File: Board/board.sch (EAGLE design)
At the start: 58 parts, among them IC1 L297, IC2 MEGA32-P, J1 +12V, Q1 BC639, Q2 BC639, Q3 BS170, Q4 BS170, Q5 BS170, Q6 BS170, X1 WATER_PUMP, X2 FAN, X3 STEP_MOT_CD, X4 STEP_MOT_AB

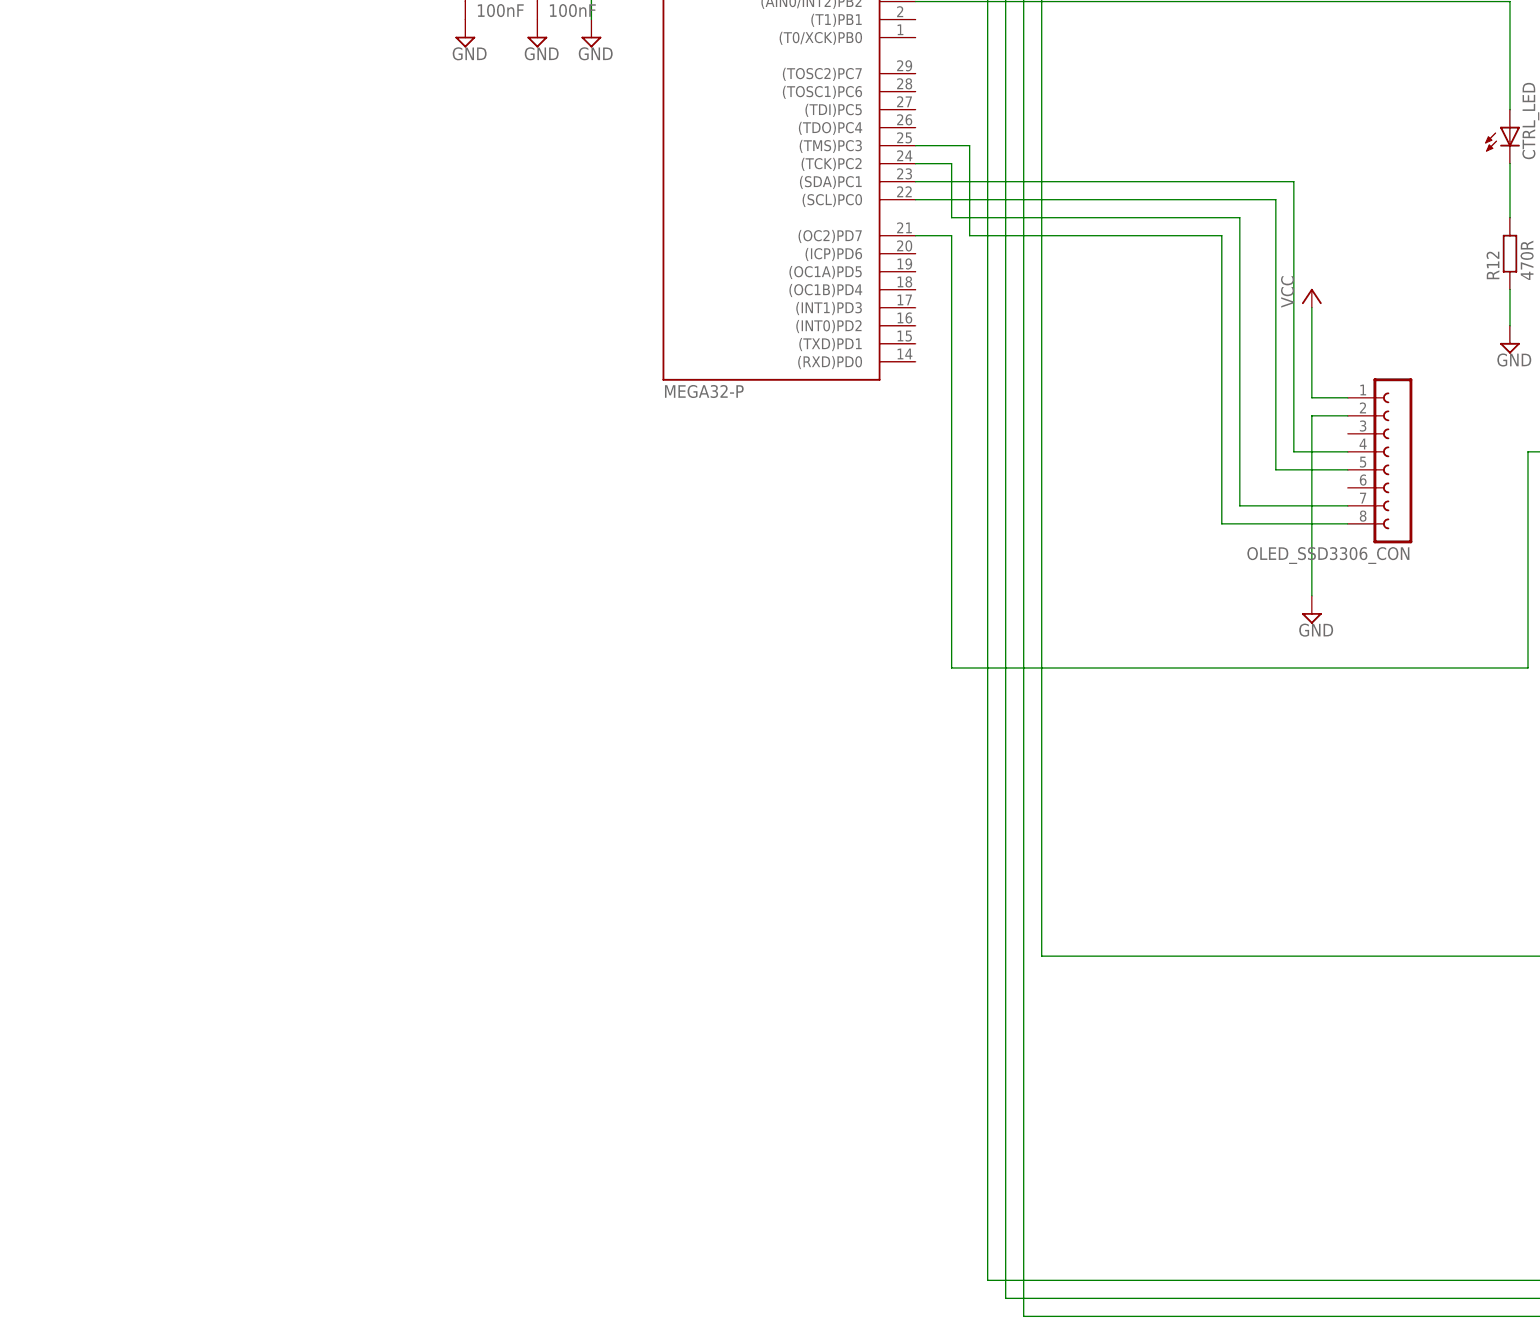
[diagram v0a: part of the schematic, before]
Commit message: mcp9808
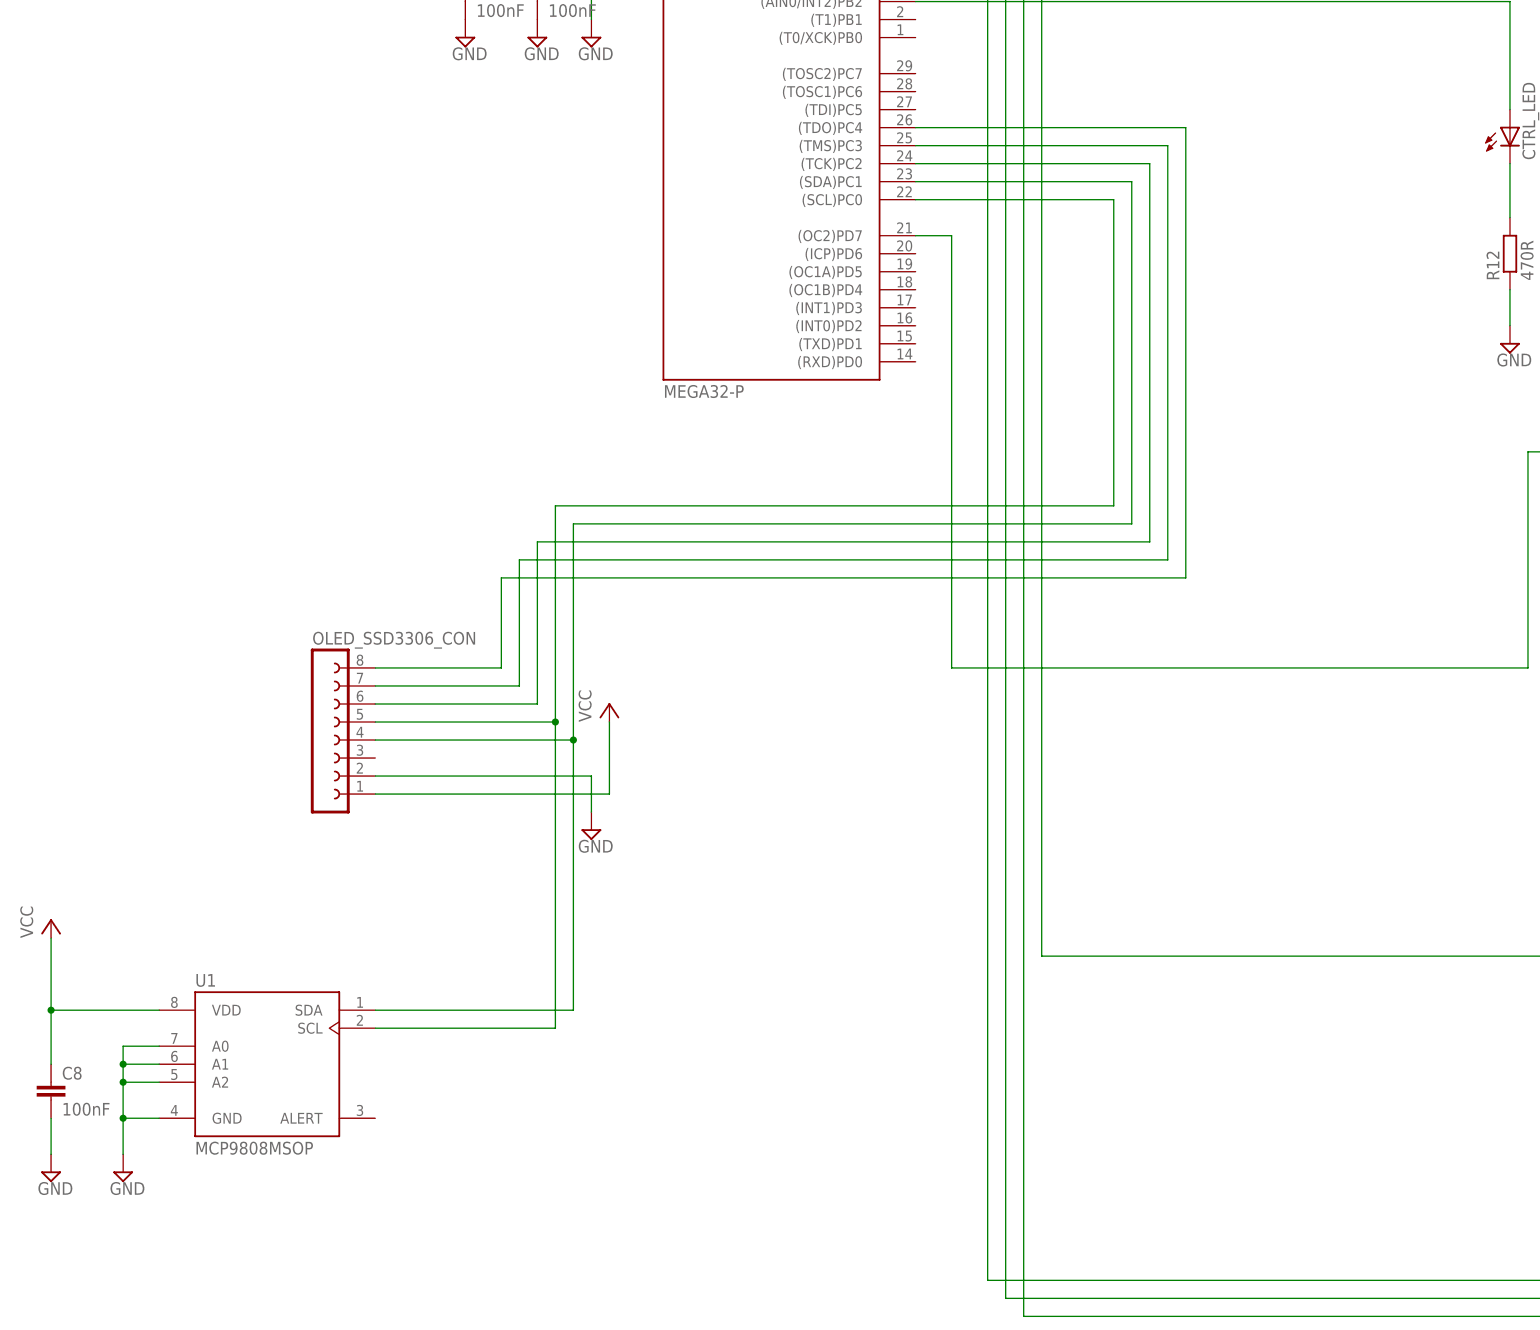
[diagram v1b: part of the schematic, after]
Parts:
- added C8: 100nF, rcl:C-EU025-025X050
- added U1: MCP9808MSOP, MCP9808:MCP9808MSOP
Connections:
- removed net OLED_RST: IC2.(TMS)PC3, OLED_SSD3306_CON.8
- removed net OLED_SA: IC2.(TCK)PC2, OLED_SSD3306_CON.7
- removed net SCL: IC2.(SCL)PC0, OLED_SSD3306_CON.5
- removed net SDA: IC2.(SDA)PC1, OLED_SSD3306_CON.4
- new net N$35: IC2.(SDA)PC1, OLED_SSD3306_CON.4, U1.SDA
- new net N$36: IC2.(SCL)PC0, OLED_SSD3306_CON.5, U1.SCL
- new net N$37: IC2.(TCK)PC2, OLED_SSD3306_CON.6
- new net N$38: IC2.(TMS)PC3, OLED_SSD3306_CON.7
- new net N$39: IC2.(TDO)PC4, OLED_SSD3306_CON.8
- net GND: now also C8.2, U1.A0, U1.A1, U1.A2, U1.GND
- net VCC: now also C8.1, U1.VDD
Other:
- moved on the sheet: OLED_SSD3306_CON

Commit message: stepper motor l298
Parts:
- removed D11: 1N5819-B, diode:1N5819-B
- removed LED1, LED2, LED3, LED4: (no value), led:LED3MM
- removed Q2: BC639, transistor-small-signal:BC639
- removed Q4, Q5, Q6: BS170, transistor-small-signal:BS170
- removed R10, R6, R8: 47K, rcl:R-EU_0207/12
- removed R11, R9: 330R, rcl:R-EU_0207/12
- removed R13, R14: 470R, rcl:R-EU_0207/12
- removed R3: (no value), rcl:R-EU_0207/12
- removed X3: STEP_MOT_CD, con-ptr500:AK500/2
- removed X4: STEP_MOT_AB, con-ptr500:AK500/2
- added IC3: L298, st-microelectronics:L298
- added X5: STEP_MOT_CD, con-ptr500:AK500/2
- added X6: STEP_MOT_AB, con-ptr500:AK500/2
- D10, D4, D5, D6, D7, D8, D9: value 1N5819-B -> 1N5824
- Q3: value BS170 -> BC639; device transistor-small-signal:BS170 -> transistor-small-signal:BC639
- R4: value 47K -> 470R
- R5: value 330R -> (none)
- R7: value 330R -> 470R
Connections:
- removed net N$11: D3.C, Q2.E, R14.2, X1-2.KL
- removed net N$14: IC1.C, Q4.G, R6.1
- removed net N$22: LED1.C, R5.2
- removed net N$24: D6.A, D7.C, Q4.D, R7.1, X4-1.KL
- removed net N$25: LED2.C, R7.2
- removed net N$30: D10.A, D11.C, Q6.D, R11.1, X3-1.KL
- removed net N$31: LED4.C, R11.2
- removed net N$32: Q3.G, R4.1
- removed net N$34: R14.1, WP_LED.A
- removed net N$5 (its old number): D2.C, Q1.E, R13.2, X2-3.KL
- removed net N$7: Q2.B, R3.2
- new net N$56: IC1.C, IC3.INPUT2
- new net N$58: IC1.B, IC3.INPUT3
- new net N$9: Q1.C, X2-1.KL
- new net VSS1: D10.C, D3.A, D4.A, D5.A, D6.A, D7.C, D8.C, D9.C, IC3.OUT1, IC3.OUT2, IC3.OUT3, IC3.OUT4, X5-1.KL, X5-2.KL, X6-1.KL, X6-2.KL
- net GND: now also D10.A, D8.A, FAN_LED.A, IC3.GND, IC3.SEN_A, IC3.SEN_B, Q1.E, Q3.E, R4.1, R7.1, WP_LED.A; no longer D11.A, D2.A, D3.A, D5.A, Q3.S, Q4.S, Q5.S, Q6.S, R10.2, R4.2, R6.2, R8.2, X1-1.KL, X2-1.KL
- net N$12: now also R5.1; no longer R3.1
- net N$13: now also IC3.INPUT1
- net N$15: now also IC1.INH1, IC3.ENABLE_A; no longer IC1.B, Q5.G, R8.1
- net N$16: now also IC3.INPUT4
- net N$21: now also IC1.INH2, IC3.ENABLE_B; no longer D4.A, D5.C, Q3.D, R5.1, X4-2.KL
- net N$27: now also FAN_LED.C, R4.2; no longer D8.A, D9.C, Q5.D, R9.1, X3-2.KL
- net N$28: now also Q3.B, R5.2; no longer LED3.C, R9.2
- net N$29: now also D2.A, Q3.C, X1-1.KL; no longer Q6.G, R10.1
- net N$33: now also R7.2, WP_LED.C; no longer FAN_LED.A, R13.1
- net VCC: now also IC3.VCC; no longer FAN_LED.C, LED1.A, LED2.A, LED3.A, LED4.A, WP_LED.C
- net VSS: now also D2.C, D3.C, D5.C, IC3.VS, X1-2.KL, X2-3.KL; no longer D10.C, D8.C, Q1.C, Q2.C
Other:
- moved on the sheet: CTRL_LED, D10, D2, D3, D4, D5, D6, D7, D8, D9, FAN_LED, KANDA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
